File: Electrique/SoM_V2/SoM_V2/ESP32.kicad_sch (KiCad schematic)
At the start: 15 parts, among them Q601 MBT3904DW1T1G, SW601 SW_BOOT, SW602 SW_CHIP_EN, U601 ESP32-S3-MINI-1U, U602 74HC238

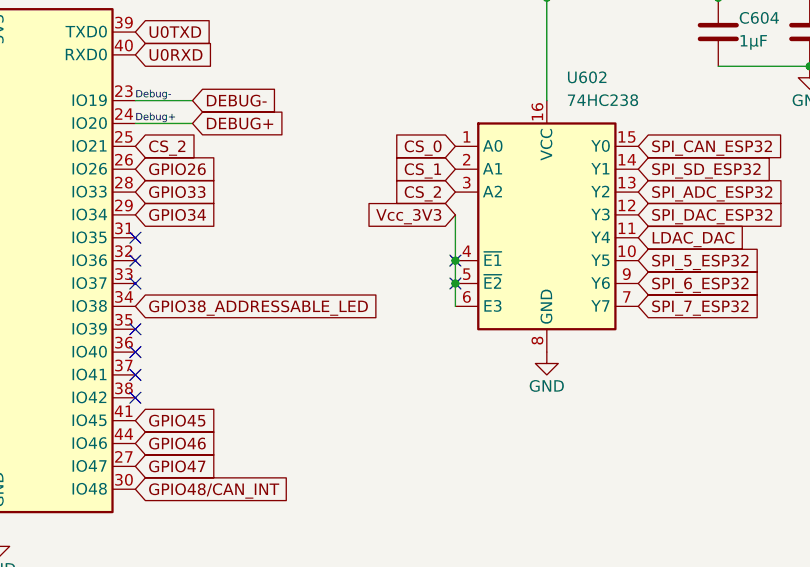
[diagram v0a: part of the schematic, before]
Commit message: push pour frank
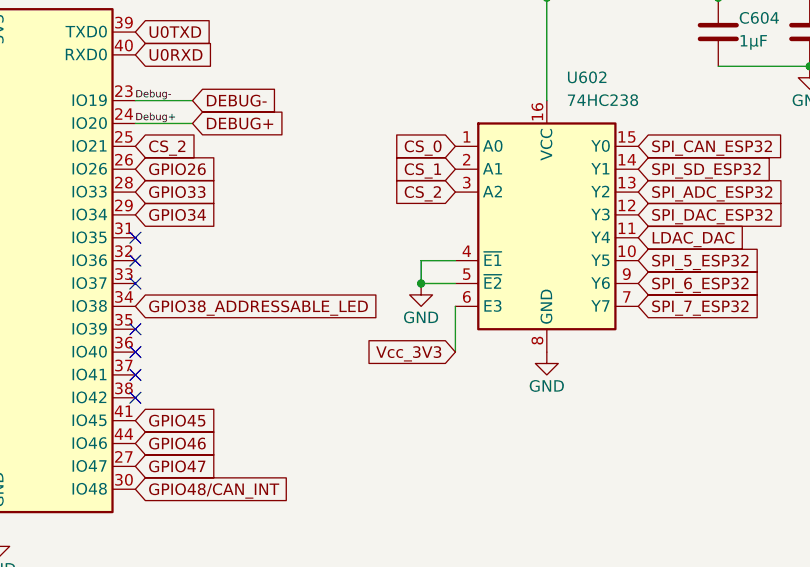
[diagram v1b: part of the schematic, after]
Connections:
- net GND: now also U602.4 (~{E1}), U602.5 (~{E2})
- net Vcc_3V3: no longer U602.4 (~{E1}), U602.5 (~{E2})
- no-connect marks 10 -> 8
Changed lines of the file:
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@@
-	)
-	(junction
-		(at 143.51 63.5)
-		(diameter 0)
-		(color 0 0 0 0)
 	)
 	(junction
@@
 	)
 	(junction
-		(at 143.51 66.04)
-		(diameter 0)
-		(color 0 0 0 0)
-	)
-	(junction
 		(at 45.72 40.64)
 		(diameter 0)
@@
 	)
 	(junction
+		(at 139.7 66.04)
+		(diameter 0)
+		(color 0 0 0 0)
+	)
+	(junction
 		(at 172.72 34.29)
 		(diameter 0)
@@
 	)
 	(no_connect
-		(at 143.51 63.5)
-	)
-	(no_connect
 		(at 107.95 60.96)
 	)
@@
 	)
 	(no_connect
-		(at 143.51 66.04)
-	)
-	(no_connect
 		(at 107.95 76.2)
 	)
@@
 	(wire
 		(pts
-			(xy 143.51 66.04) (xy 143.51 68.58)
-		)
-		(stroke
-			(width 0)
-			(type default)
-		)
-	)
-	(wire
-		(pts
 			(xy 30.48 40.64) (xy 30.48 45.72)
 		)
@@
 	(wire
 		(pts
+			(xy 139.7 66.04) (xy 143.51 66.04)
+		)
+		(stroke
+			(width 0)
+			(type default)
+		)
+	)
+	(wire
+		(pts
 			(xy 114.3 48.26) (xy 107.95 48.26)
 		)
@@
 	(wire
 		(pts
+			(xy 139.7 63.5) (xy 139.7 66.04)
+		)
+		(stroke
+			(width 0)
+			(type default)
+		)
+	)
+	(wire
+		(pts
 			(xy 271.78 91.44) (xy 271.78 82.55)
 		)
@@
 	(wire
 		(pts
+			(xy 143.51 63.5) (xy 139.7 63.5)
+		)
+		(stroke
+			(width 0)
+			(type default)
+		)
+	)
+	(wire
+		(pts
 			(xy 92.71 22.86) (xy 92.71 29.21)
 		)
@@
 	(wire
 		(pts
-			(xy 143.51 58.42) (xy 143.51 63.5)
+			(xy 143.51 73.66) (xy 143.51 68.58)
 		)
 		(stroke
@@
 		(pts
 			(xy 172.72 41.91) (xy 182.88 41.91)
-		)
-		(stroke
-			(width 0)
-			(type default)
-		)
-	)
-	(wire
-		(pts
-			(xy 143.51 63.5) (xy 143.51 66.04)
 		)
 		(stroke
@@
 	(global_label "Vcc_3V3"
 		(shape input)
-		(at 143.51 58.42 180)
+		(at 143.51 73.66 180)
 		(fields_autoplaced yes)
 		(effects
@@
 		)
 		(property "Intersheetrefs" "${INTERSHEET_REFS}"
-			(at 132.7838 58.42 0)
+			(at 132.7838 73.66 0)
 			(effects
 				(font
@@
 					(unit 1)
 				)
+			)
+		)
+	)
+	(symbol
+		(lib_id "power:GND")
+		(at 139.7 66.04 0)
+		(unit 1)
+		(exclude_from_sim no)
+		(in_bom yes)
+		(on_board yes)
+		(dnp no)
+		(property "Reference" "#PWR0608"
+			(at 139.7 72.39 0)
+			(effects
+				(font
+					(size 1.27 1.27)
+				)
+				(hide yes)
+			)
+		)
+		(property "Value" "GND"
+			(at 139.7 69.85 0)
+			(effects
+				(font
+					(size 1.27 1.27)
+				)
+			)
+		)
+		(property "Footprint" ""
+			(at 139.7 66.04 0)
+			(effects
+				(font
+					(size 1.27 1.27)
+				)
+				(hide yes)
+			)
+		)
+		(property "Datasheet" ""
+			(at 139.7 66.04 0)
+			(effects
+				(font
+					(size 1.27 1.27)
+				)
+				(hide yes)
+			)
+		)
+		(property "Description" "Power symbol creates a global label with name \"GND\" , ground"
+			(at 139.7 66.04 0)
+			(effects
+				(font
+					(size 1.27 1.27)
+				)
+				(hide yes)
+			)
+		)
+		(pin "1"
+		)
+		(instances
+			(project "SoM_V2"
+				(path "/ecd44d9a-8113-48e2-a5bb-0de07ce8b9ce/42eddecc-5d06-4740-ba8f-a05813435351"
+					(reference "#PWR0608")
+					(unit 1)
+				)

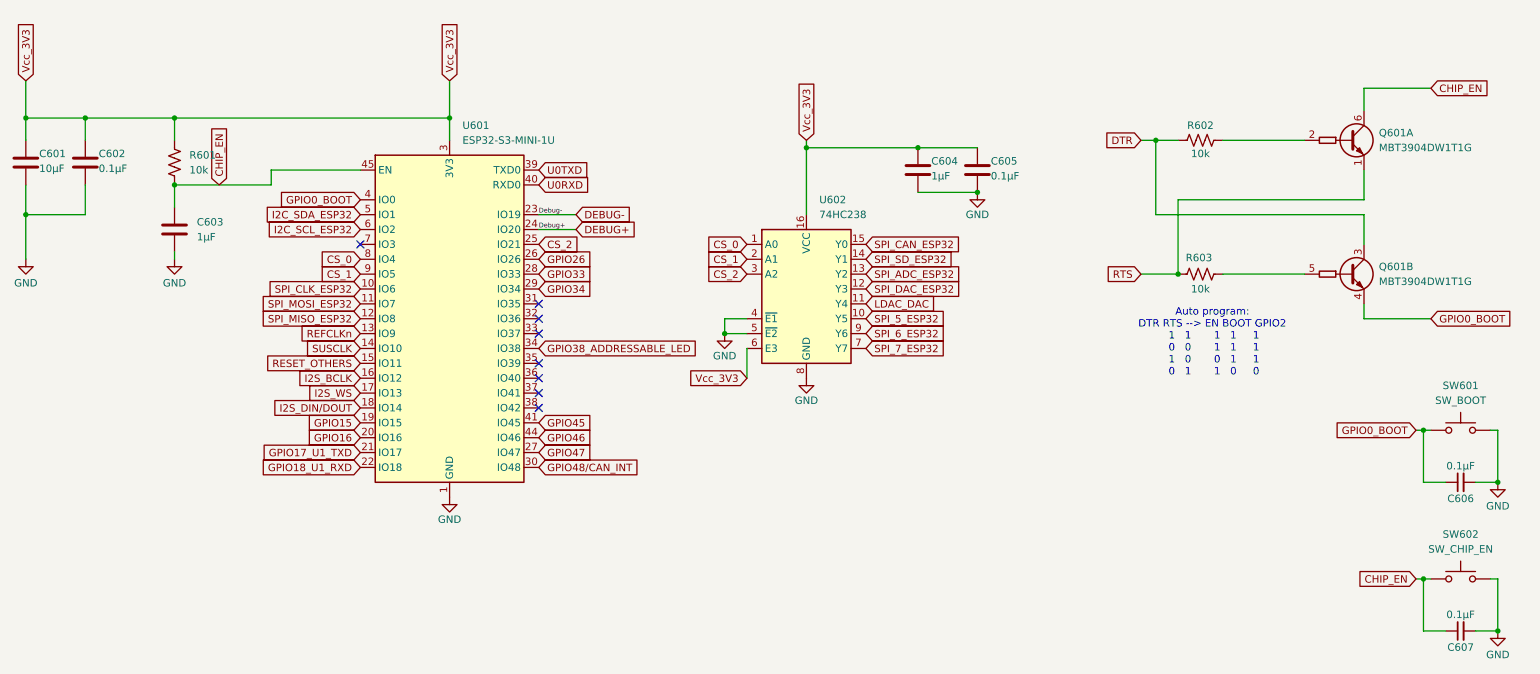
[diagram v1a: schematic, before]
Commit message: push fix ???
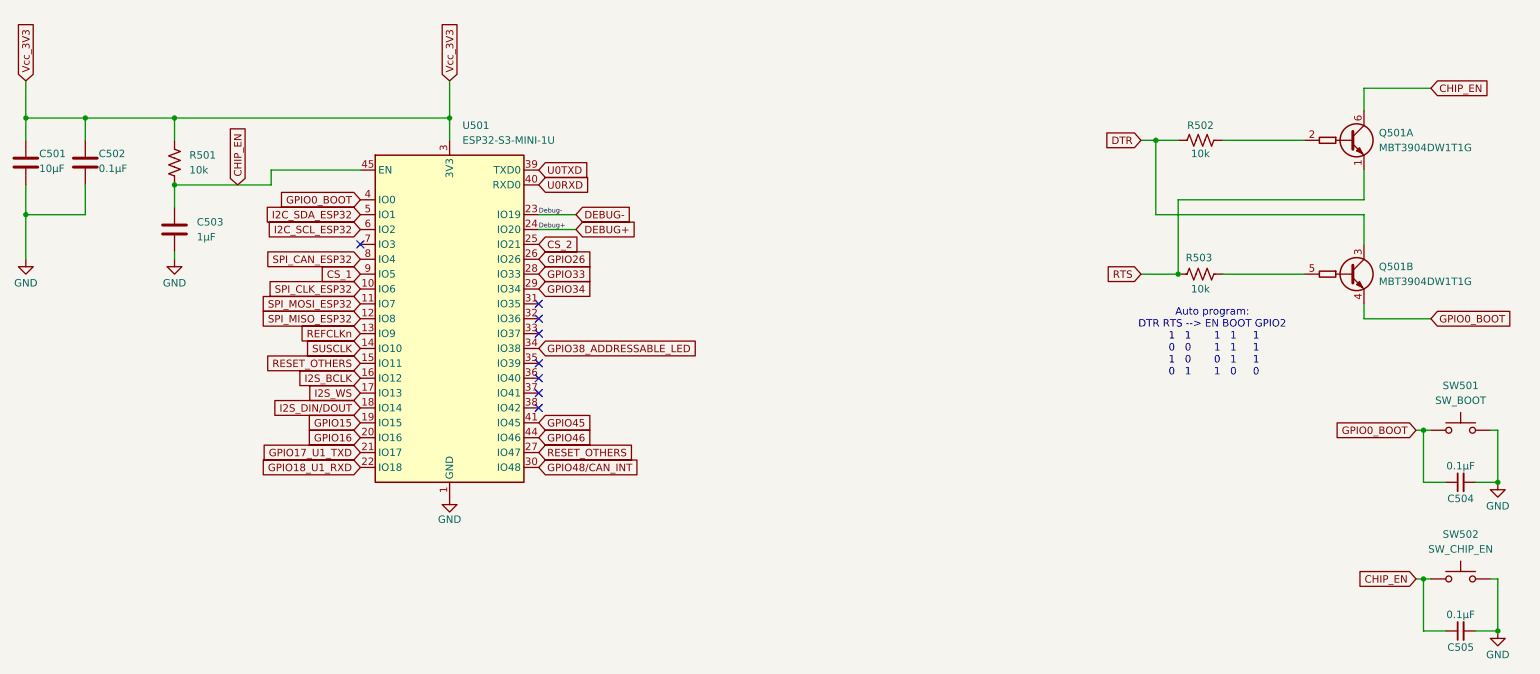
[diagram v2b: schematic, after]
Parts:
- removed C604: 1µF, Resistor_SMD:R_0805_2012Metric, symbol Device:C
- removed C605: 0.1µF, Resistor_SMD:R_0805_2012Metric, symbol Device:C
- removed U602: 74HC238, Package_DFN_QFN:DHVQFN-16-1EP_2.5x3.5mm_P0.5mm_EP1x2mm, symbol 74xx:74HC238
- renumbered C601 to C501, C602 to C502, C603 to C503, C606 to C504, C607 to C505, Q601 to Q501, R601 to R501, R602 to R502, R603 to R503, SW601 to SW501, SW602 to SW502, U601 to U501
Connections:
- net CS_0 is gone; now on net SPI_CAN_ESP32: U501.8 (IO4)
- net GPIO47 is gone; now on net RESET_OTHERS: U501.27 (IO47)

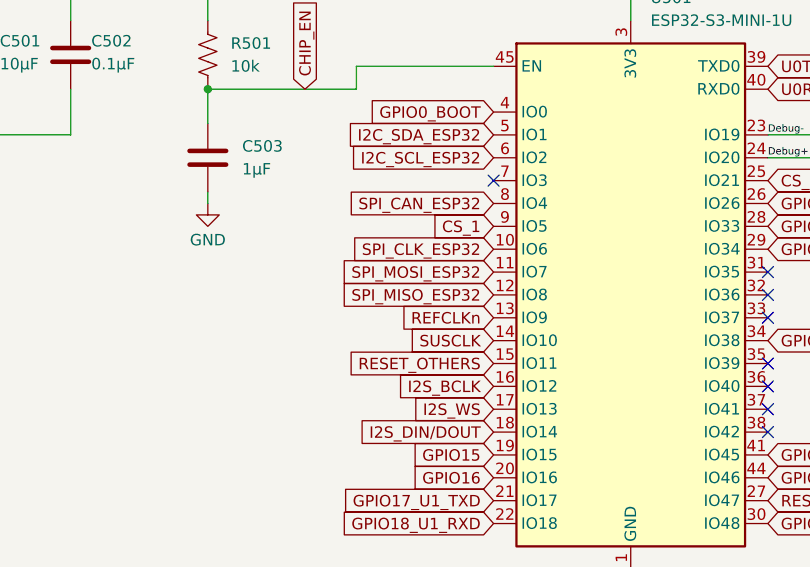
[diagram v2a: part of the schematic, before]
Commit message: push v2.2
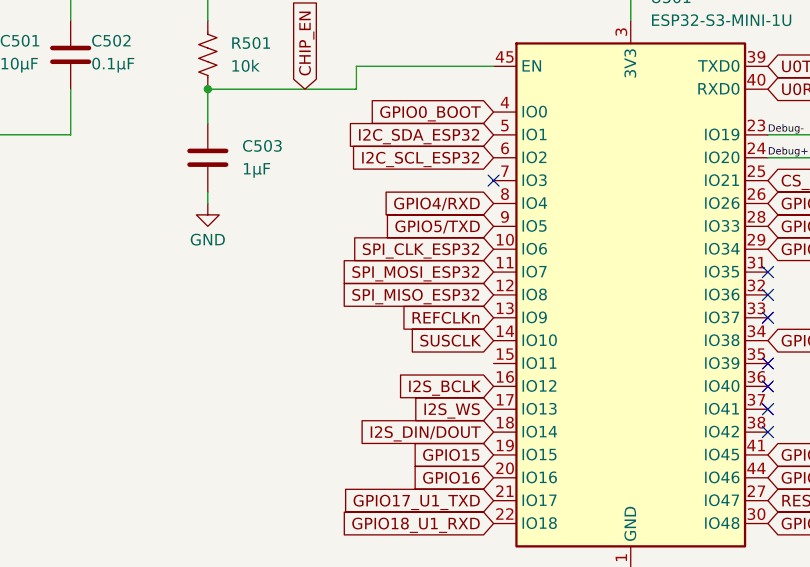
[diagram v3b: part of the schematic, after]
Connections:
- net RESET_OTHERS: no longer U501.15 (IO11)
- net CS_1 renamed GPIO5/TXD
- net SPI_CAN_ESP32 renamed GPIO4/RXD
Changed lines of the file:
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@@
 		)
 	)
-	(global_label "RESET_OTHERS"
-		(shape input)
-		(at 77.47 71.12 180)
-		(fields_autoplaced yes)
-		(effects
-			(font
-				(size 1.27 1.27)
-			)
-			(justify right)
-		)
-		(property "Intersheetrefs" "${INTERSHEET_REFS}"
-			(at 60.515 71.12 0)
+	(global_label "GPIO4{slash}RXD"
+		(shape input)
+		(at 77.47 53.34 180)
+		(fields_autoplaced yes)
+		(effects
+			(font
+				(size 1.27 1.27)
+			)
+			(justify right)
+		)
+		(property "Intersheetrefs" "${INTERSHEET_REFS}"
+			(at 63.72 53.34 0)
 			(effects
 				(font
@@
 		)
 	)
-	(global_label "CS_1"
+	(global_label "GPIO5{slash}TXD"
 		(shape input)
 		(at 77.47 55.88 180)
@@
 		)
 		(property "Intersheetrefs" "${INTERSHEET_REFS}"
-			(at 69.8282 55.88 0)
+			(at 64.0224 55.88 0)
 			(effects
 				(font
@@
 				(hide yes)
 			)
-		)
-	)
-	(global_label "SPI_CAN_ESP32"
-		(shape input)
-		(at 77.47 53.34 180)
-		(fields_autoplaced yes)
-		(effects
-			(font
-				(size 1.27 1.27)
-			)
-			(justify right)
-		)
-		(property "Intersheetrefs" "${INTERSHEET_REFS}"
-			(at 59.7287 53.34 0)
-			(effects
-				(font
-					(size 1.27 1.27)
-				)
-				(justify right)
-				(hide yes)
-			)
